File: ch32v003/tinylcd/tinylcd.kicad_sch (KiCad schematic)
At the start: 5 parts, among them U1 RB017A1505A_Connector

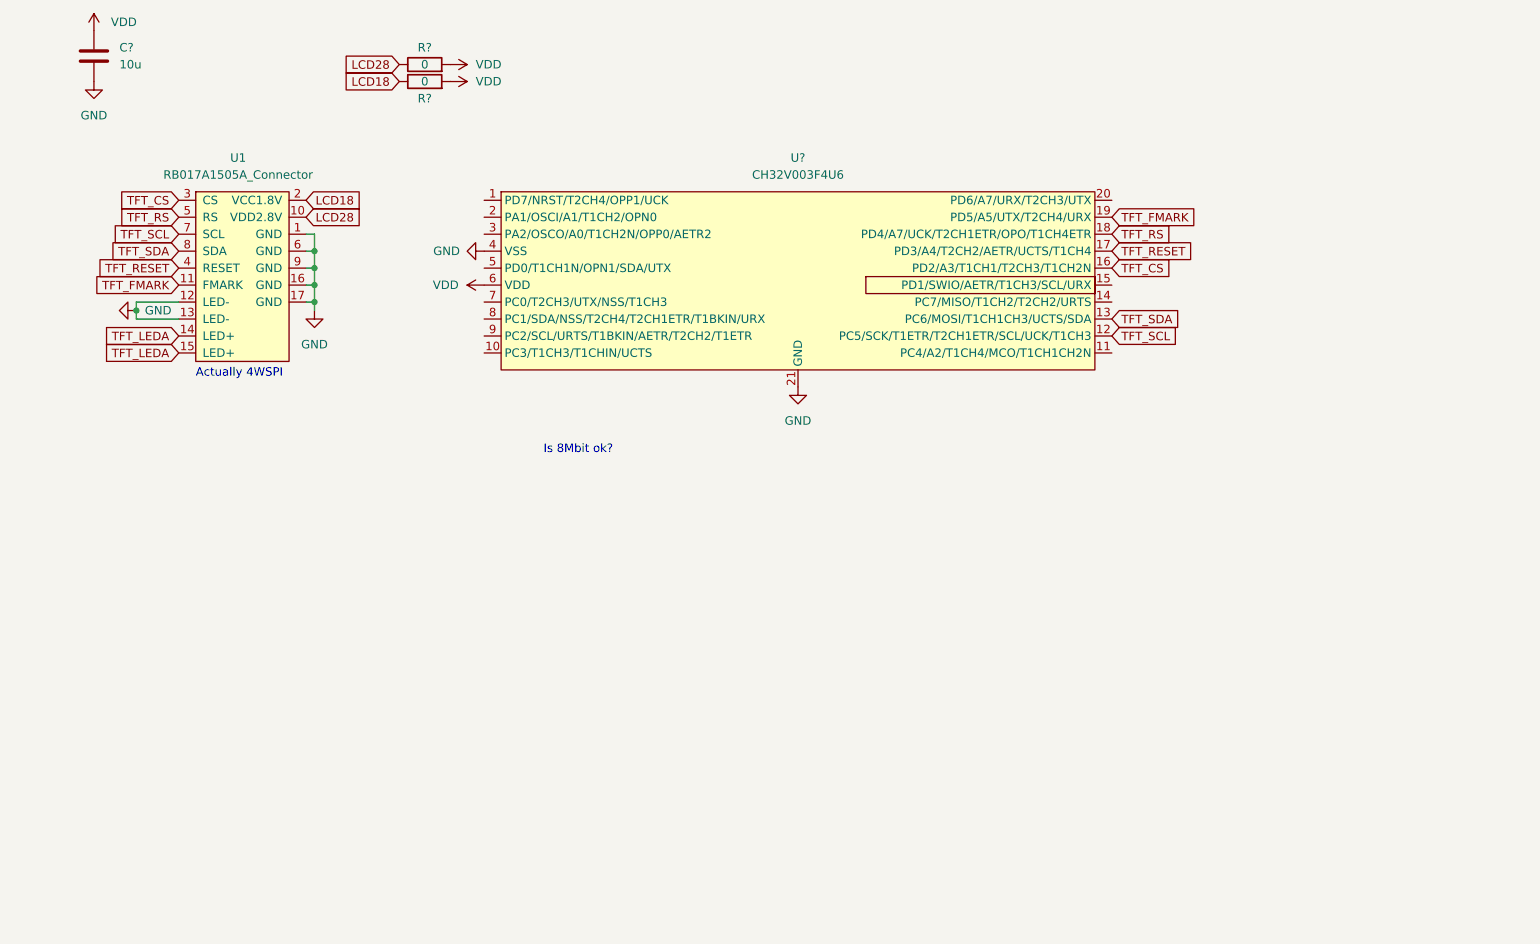
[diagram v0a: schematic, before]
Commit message: Bump versions.
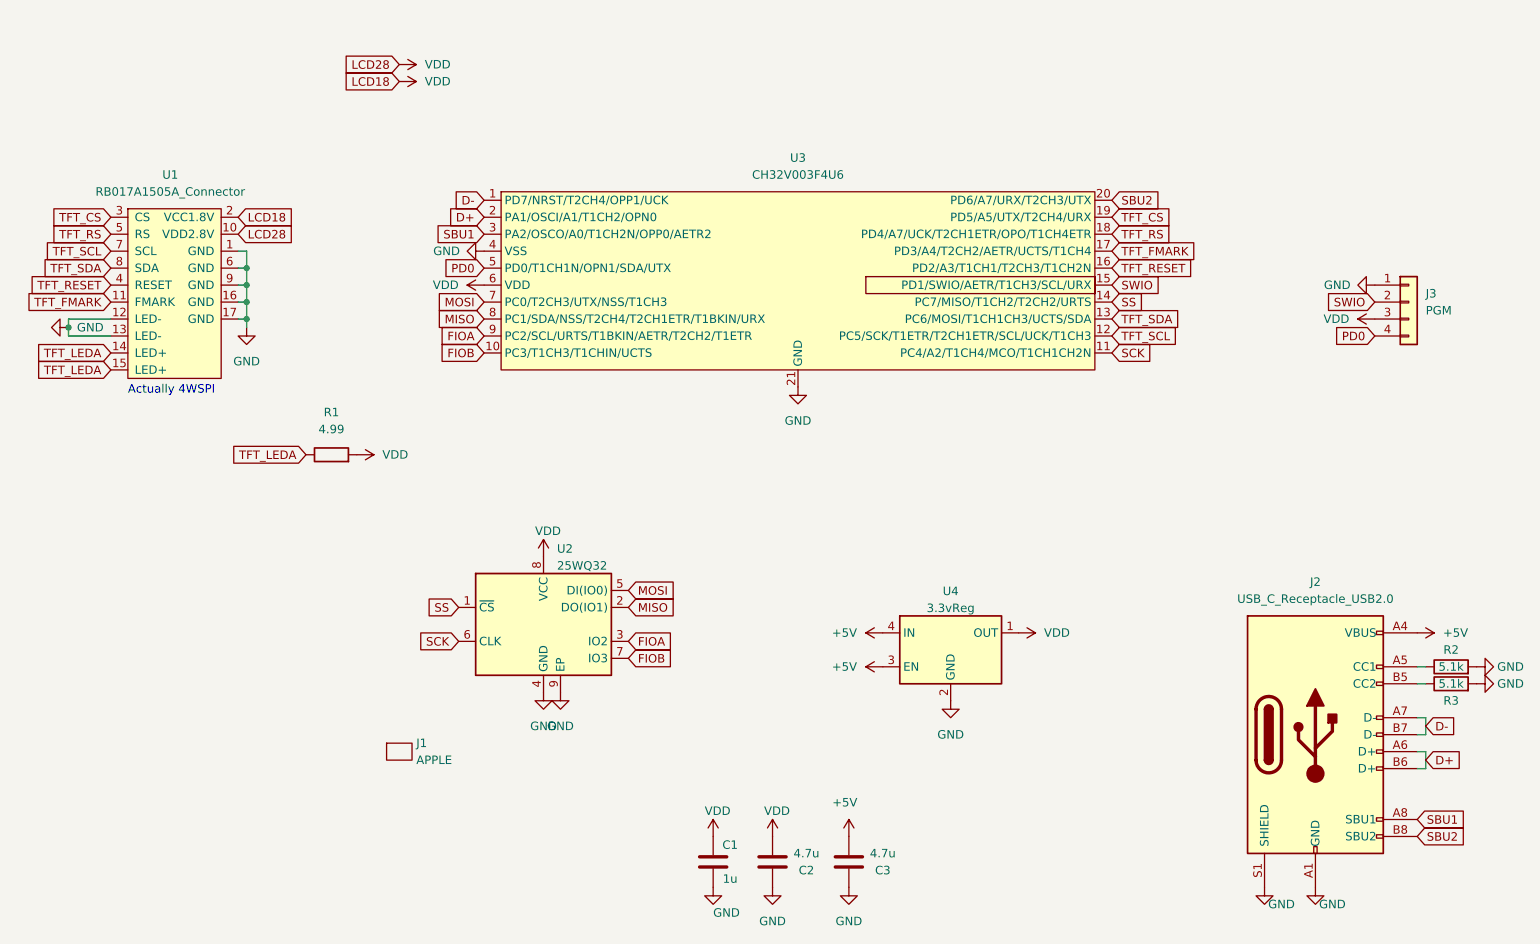
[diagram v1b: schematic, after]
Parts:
- removed C?: 10u, Capacitor_SMD:C_0402_1005Metric, symbol Device:C
- removed R? (x2): 0, Resistor_SMD:R_0402_1005Metric, symbol Device:R
- added C1: 1u, Resistor_SMD:R_0402_1005Metric, symbol Device:C
- added C2, C3: 4.7u, Resistor_SMD:R_0402_1005Metric, symbol Device:C
- added J1: APPLE, artwork:apple, symbol artwork:artwork
- added J2: USB_C_Receptacle_USB2.0, Connector_USB:USB_C_Receptacle_HRO_TYPE-C-31-M-12, symbol Connector:USB_C_Receptacle_USB2.0
- added J3: PGM, Connector_PinHeader_2.54mm:PinHeader_1x04_P2.54mm_Vertical, symbol Connector_Generic:Conn_01x04
- added R1: 4.99, Resistor_SMD:R_0603_1608Metric, symbol Device:R
- added R2, R3: 5.1k, Resistor_SMD:R_0402_1005Metric, symbol Device:R
- added U2: 25WQ32, cnhardware:USON8-LINE(2x3), symbol Memory_Flash:W25Q32JVZP
- added U4: 3.3vReg, cnhardware:xdfn-reg, symbol Regulator_Linear:NCP115AMX120TCG
- gave numbers to parts that had none: 1
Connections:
- net LCD18 is gone; now on net VDD: U1.2 (VCC1.8V)
- net LCD28 is gone; now on net VDD: U1.10 (VDD2.8V)
- net GND: now also C1.1, C2.1, C3.1, J2.A1 (GND), J2.A12 (GND), J2.B1 (GND), J2.B12 (GND), J2.S1 (SHIELD), J3.1 (Pin_1), R2.2, R3.2, U2.4 (GND), U2.9 (EP), U4.2 (GND), U4.5 (GND)
- net TFT_CS: now also U3.19 (PD5/A5/UTX/T2CH4/URX); no longer U3.16 (PD2/A3/T1CH1/T2CH3/T1CH2N)
- net TFT_FMARK: now also U3.17 (PD3/A4/T2CH2/AETR/UCTS/T1CH4); no longer U3.19 (PD5/A5/UTX/T2CH4/URX)
- net TFT_LEDA: now also R1.1
- net TFT_RESET: now also U3.16 (PD2/A3/T1CH1/T2CH3/T1CH2N); no longer U3.17 (PD3/A4/T2CH2/AETR/UCTS/T1CH4)
- net VDD: now also C1.2, C2.2, J3.3 (Pin_3), R1.2, U2.8 (VCC), U4.1 (OUT)
- net D-: now reaches U3.1 (PD7/NRST/T2CH4/OPP1/UCK)
- net D-: now also J2.A7 (D-), J2.B7 (D-)
- net FIOB: now reaches U3.10 (PC3/T1CH3/T1CHIN/UCTS)
- net FIOB: now also U2.7 (IO3)
- net SCK: now reaches U3.11 (PC4/A2/T1CH4/MCO/T1CH1CH2N)
- net SCK: now also U2.6 (CLK)
- net SS: now reaches U3.14 (PC7/MISO/T1CH2/T2CH2/URTS)
- net SS: now also U2.1 (~{CS})
- net SWIO: now reaches U3.15 (PD1/SWIO/AETR/T1CH3/SCL/URX)
- net SWIO: now also J3.2 (Pin_2)
- net D+: now reaches U3.2 (PA1/OSCI/A1/T1CH2/OPN0)
- net D+: now also J2.A6 (D+), J2.B6 (D+)
- net SBU2: now reaches U3.20 (PD6/A7/URX/T2CH3/UTX)
- net SBU2: now also J2.B8 (SBU2)
- net SBU1: now reaches U3.3 (PA2/OSCO/A0/T1CH2N/OPP0/AETR2)
- net SBU1: now also J2.A8 (SBU1)
- net PD0: now reaches U3.5 (PD0/T1CH1N/OPN1/SDA/UTX)
- net PD0: now also J3.4 (Pin_4)
- net MOSI: now reaches U3.7 (PC0/T2CH3/UTX/NSS/T1CH3)
- net MOSI: now also U2.5 (DI(IO0))
- net MISO: now reaches U3.8 (PC1/SDA/NSS/T2CH4/T2CH1ETR/T1BKIN/URX)
- net MISO: now also U2.2 (DO(IO1))
- net FIOA: now reaches U3.9 (PC2/SCL/URTS/T1BKIN/AETR/T2CH2/T1ETR)
- net FIOA: now also U2.3 (IO2)
- new net: J2.B5 (CC2), R3.1
- new net: J2.A5 (CC1), R2.1
- new net +5V: C3.2, J2.A4 (VBUS), J2.A9 (VBUS), J2.B4 (VBUS), J2.B9 (VBUS), U4.3 (EN), U4.4 (IN)
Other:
- note removed: "Is 8Mbit ok?"
- moved on the sheet: U1
